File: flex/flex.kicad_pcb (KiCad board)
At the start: 2 copper layers, 126.3 x 91.6 mm, 91 parts, among them J1 Conn_01x04_Female, J2 Conn_01x05_Female, J3 Conn_01x03_Female, J4 Conn_01x06_Female, J5 Conn_01x03_Female, SW10 SW_Push, SW11 SW_Push, SW12 SW_Push, SW15 SW_Push, SW16 SW_Push, SW17 SW_Push, SW2 SW_Push, SW20 SW_Push, SW21 SW_Push, SW22 SW_Push, SW24 SW_Push, SW25 SW_Push, SW26 SW_Push, SW3 SW_Push, SW4 SW_Push, SW6 SW_Push, SW7 SW_Push, SW8 SW_Push

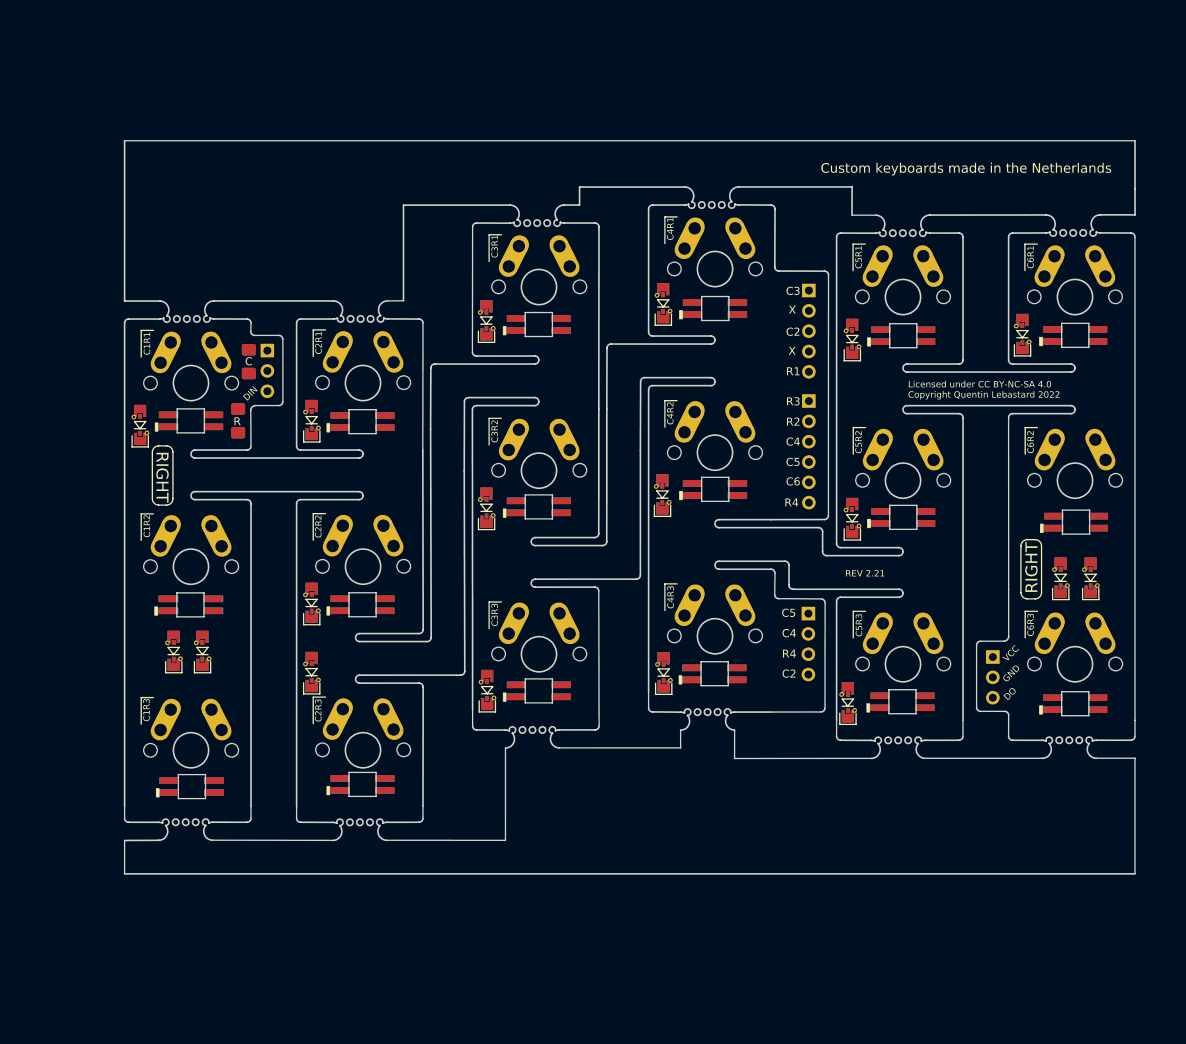
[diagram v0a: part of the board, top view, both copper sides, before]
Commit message: routing
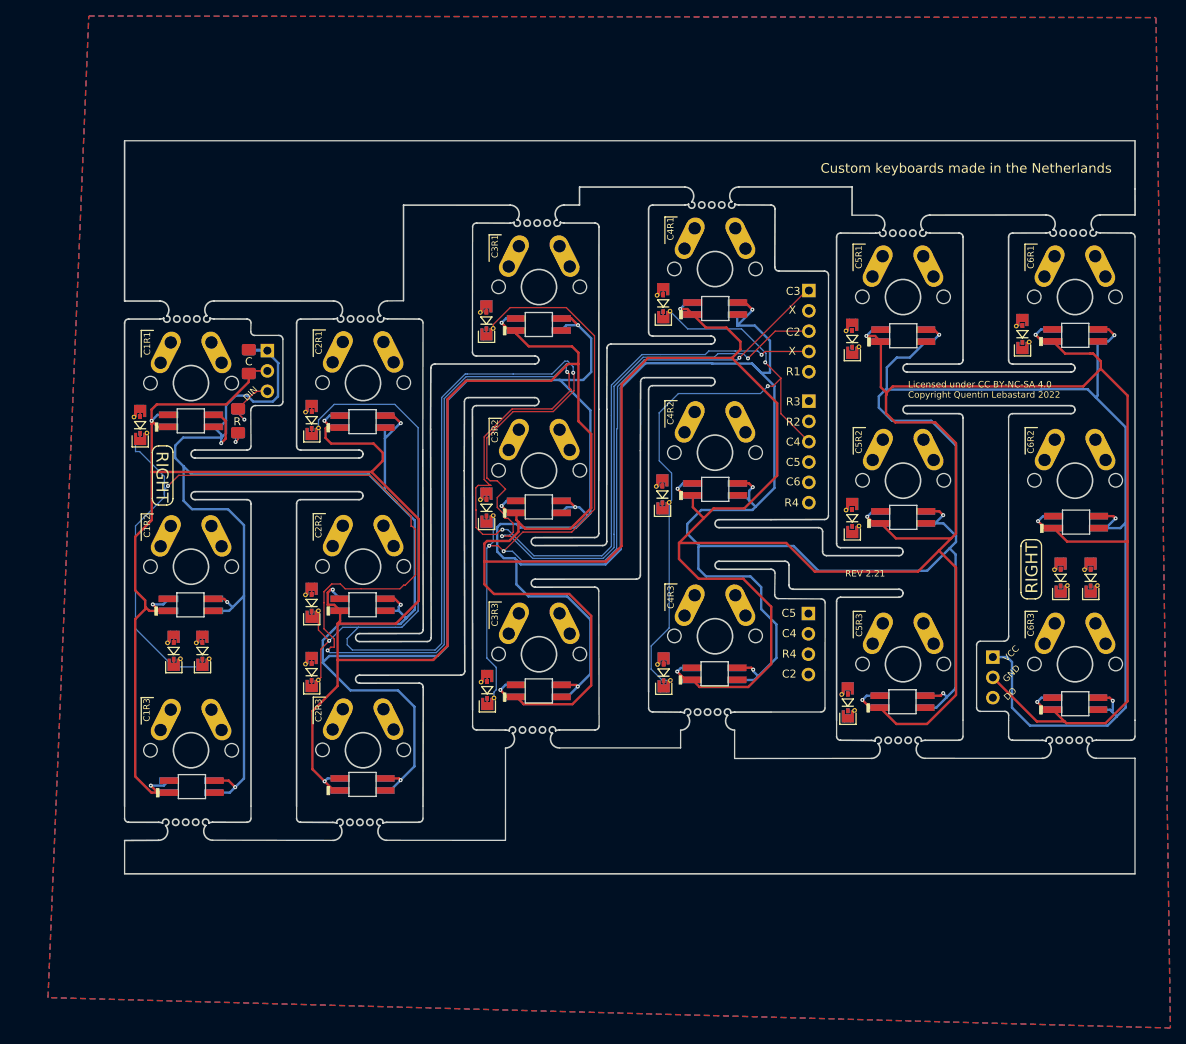
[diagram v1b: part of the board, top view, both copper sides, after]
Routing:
- net Gnd: track 0.00 -> 754.7 mm, vias 0 -> 18
- net Vcc: track 0.00 -> 725.8 mm, vias 0 -> 18
- net col1: track 0.00 -> 265.9 mm, vias 0 -> 5
- net col2: track 0.00 -> 227.6 mm, vias 0 -> 4
- net col3: track 0.00 -> 146.7 mm, vias 0 -> 3
- net col4: track 0.00 -> 87.0 mm, vias 0 -> 2
- net Din: track 0.00 -> 7.91 mm, vias 0 -> 1
- net Net-(D28-DIN): track 0.00 -> 2.57 mm, vias 0 -> 1
- net Net-(D9-A): track 0.00 -> 1.92 mm
- net Net-(D27-A): track 0.00 -> 1.92 mm
- net Net-(D20-A): track 0.00 -> 1.92 mm
- net Net-(D2-A): track 0.00 -> 1.92 mm
- net Net-(D19-A): track 0.00 -> 1.92 mm
- net Net-(D15-A): track 0.00 -> 1.92 mm
- net Net-(D13-A): track 0.00 -> 1.92 mm
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- added copper zone on B.Cu, net Gnd
- added copper zone on F.Cu, net Gnd

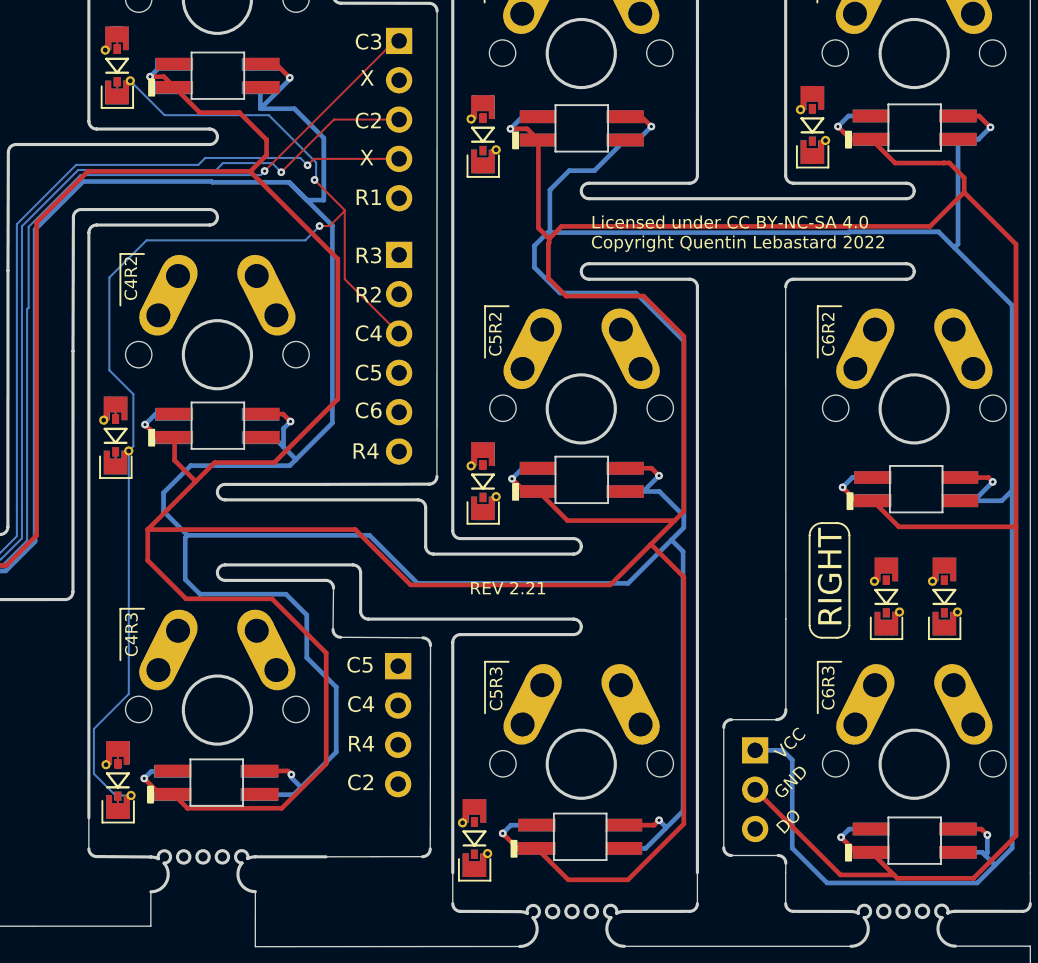
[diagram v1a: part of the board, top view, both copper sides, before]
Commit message: routing
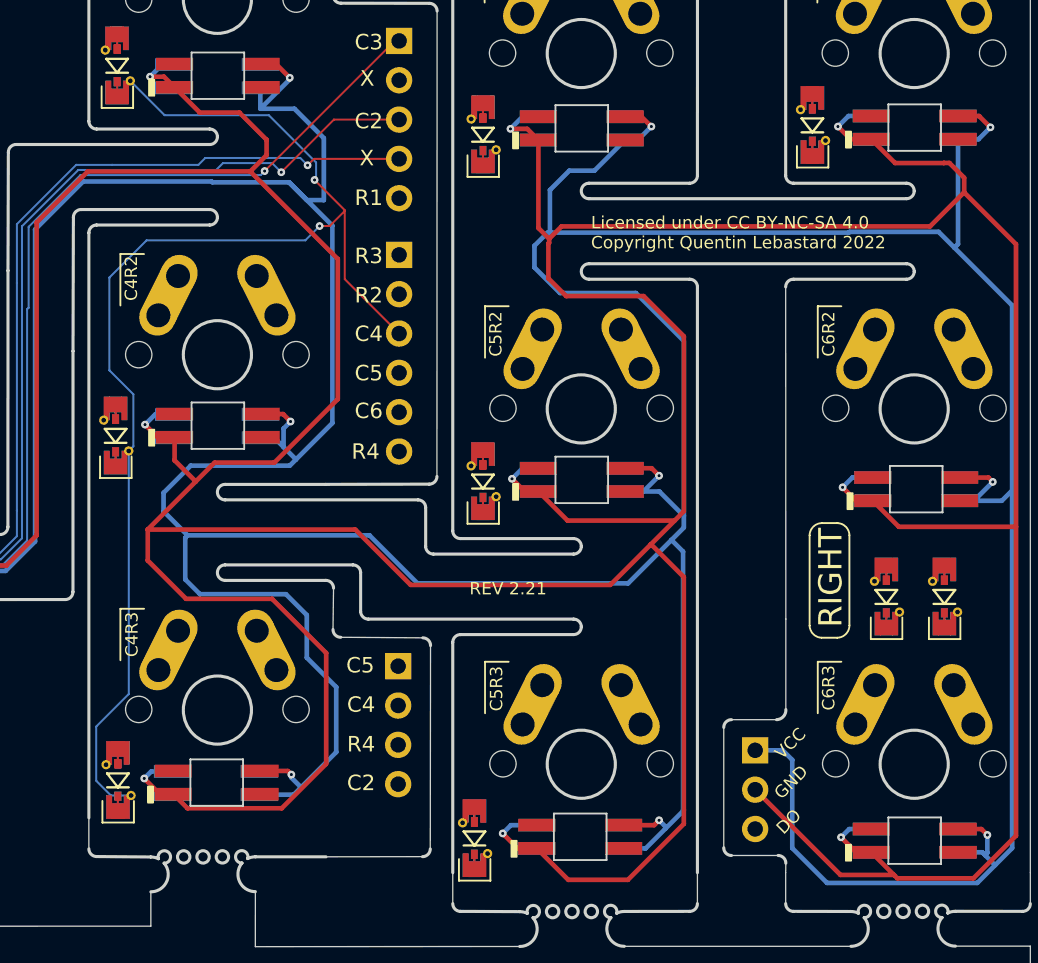
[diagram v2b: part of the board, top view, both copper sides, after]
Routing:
- net col6: track 0.00 -> 5.75 mm
- net col5: track 0.00 -> 5.75 mm
- net Net-(D36-A): track 0.00 -> 1.92 mm
- net Net-(D35-A): track 0.00 -> 1.92 mm
- net Net-(D32-A): track 0.00 -> 1.92 mm
- net Net-(D31-A): track 0.00 -> 1.92 mm
- net Net-(D16-A): track 0.00 -> 1.92 mm
- net Net-(D14-A): track 0.00 -> 1.92 mm
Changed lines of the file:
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@@
-	)
-	(segment
-		(start 101.25 114.05)
-		(end 102.65 115.45)
-		(width 0.13)
-		(layer "B.Cu")
-		(net 9)
 	)
 	(segment
@@
 	)
 	(segment
-		(start 103.5 108.9)
-		(end 101.25 111.15)
-		(width 0.13)
-		(layer "B.Cu")
-		(net 9)
-	)
-	(segment
 		(start 115.6 74.57168)
 		(end 115.6 75.6)
@@
 	)
 	(segment
+		(start 102.35 115.45)
+		(end 103.65 115.45)
+		(width 0.13)
+		(layer "B.Cu")
+		(net 9)
+	)
+	(segment
+		(start 103.5 108.9)
+		(end 101.4 111)
+		(width 0.13)
+		(layer "B.Cu")
+		(net 9)
+	)
+	(segment
+		(start 104.65 79.6)
+		(end 114.9 79.6)
+		(width 0.13)
+		(layer "B.Cu")
+		(net 9)
+	)
+	(segment
+		(start 101.4 111)
+		(end 101.4 114.5)
+		(width 0.13)
+		(layer "B.Cu")
+		(net 9)
+	)
+	(segment
 		(start 103.5 93.2)
 		(end 103.5 108.9)
@@
 	)
 	(segment
-		(start 104.65 79.6)
-		(end 114.9 79.6)
-		(width 0.13)
-		(layer "B.Cu")
-		(net 9)
-	)
-	(segment
-		(start 101.25 111.15)
-		(end 101.25 114.05)
-		(width 0.13)
-		(layer "B.Cu")
-		(net 9)
-	)
-	(segment
-		(start 102.65 115.45)
-		(end 103.65 115.45)
-		(width 0.13)
-		(layer "B.Cu")
-		(net 9)
-	)
-	(segment
 		(start 114.9 79.6)
 		(end 115.825735 78.674265)
@@
 		(layer "B.Cu")
 		(net 9)
+	)
+	(segment
+		(start 101.4 114.5)
+		(end 102.35 115.45)
+		(width 0.13)
+		(layer "B.Cu")
+		(net 9)
+	)
+	(segment
+		(start 125.8252 120.2105)
+		(end 125.8252 119.25275)
+		(width 0.13)
+		(layer "F.Cu")
+		(net 13)
+	)
+	(segment
+		(start 126.3752 73.80275)
+		(end 126.3752 74.7605)
+		(width 0.13)
+		(layer "F.Cu")
+		(net 13)
+	)
+	(segment
+		(start 126.3752 97.1605)
+		(end 126.3752 96.20275)
+		(width 0.13)
+		(layer "F.Cu")
+		(net 13)
+	)
+	(segment
+		(start 125.8252 120.2105)
+		(end 125.8252 119.25275)
+		(width 0.13)
+		(layer "B.Cu")
+		(net 13)
+	)
+	(segment
+		(start 126.3752 73.80275)
+		(end 126.3752 74.7605)
+		(width 0.13)
+		(layer "B.Cu")
+		(net 13)
+	)
+	(segment
+		(start 126.3752 96.20275)
+		(end 126.3752 97.1605)
+		(width 0.13)
+		(layer "B.Cu")
+		(net 13)
+	)
+	(segment
+		(start 147.65 74.15775)
+		(end 147.65 73.2)
+		(width 0.13)
+		(layer "F.Cu")
+		(net 14)
+	)
+	(segment
+		(start 152.4252 104.6105)
+		(end 152.4252 103.65275)
+		(width 0.13)
+		(layer "F.Cu")
+		(net 14)
+	)
+	(segment
+		(start 156.1752 104.6105)
+		(end 156.1752 103.65275)
+		(width 0.13)
+		(layer "F.Cu")
+		(net 14)
+	)
+	(segment
+		(start 156.1752 104.6105)
+		(end 156.1752 103.65275)
+		(width 0.13)
+		(layer "B.Cu")
+		(net 14)
+	)
+	(segment
+		(start 152.4252 103.65275)
+		(end 152.4252 104.6105)
+		(width 0.13)
+		(layer "B.Cu")
+		(net 14)
+	)
+	(segment
+		(start 147.65 73.2)
+		(end 147.65 74.15775)
+		(width 0.13)
+		(layer "B.Cu")
+		(net 14)
 	)
 	(segment
@@
 	)
 	(segment
+		(start 126.3752 71.70275)
+		(end 126.3752 70.745)
+		(width 0.13)
+		(layer "F.Cu")
+		(net 25)
+	)
+	(segment
+		(start 126.3752 70.745)
+		(end 126.3752 71.70275)
+		(width 0.13)
+		(layer "B.Cu")
+		(net 25)
+	)
+	(segment
 		(start 58.8 104.7)
 		(end 58.8 103.74225)
@@
 	)
 	(segment
+		(start 147.65 71.1)
+		(end 147.65 70.14225)
+		(width 0.13)
+		(layer "F.Cu")
+		(net 27)
+	)
+	(segment
+		(start 147.65 70.14225)
+		(end 147.65 71.1)
+		(width 0.13)
+		(layer "B.Cu")
+		(net 27)
+	)
+	(segment
 		(start 80.75 115.6)
 		(end 80.75 114.64225)
@@
 	)
 	(segment
+		(start 125.8252 117.15275)
+		(end 125.8252 116.195)
+		(width 0.13)
+		(layer "F.Cu")
+		(net 36)
+	)
+	(segment
+		(start 125.8252 117.15275)
+		(end 125.8252 116.195)
+		(width 0.13)
+		(layer "B.Cu")
+		(net 36)
+	)
+	(segment
+		(start 126.3752 94.10275)
+		(end 126.3752 93.145)
+		(width 0.13)
+		(layer "F.Cu")
+		(net 37)
+	)
+	(segment
+		(start 126.3752 93.145)
+		(end 126.3752 94.10275)
+		(width 0.13)
+		(layer "B.Cu")
+		(net 37)
+	)
+	(segment
+		(start 156.1752 101.55275)
+		(end 156.1752 100.595)
+		(width 0.13)
+		(layer "F.Cu")
+		(net 38)
+	)
+	(segment
+		(start 156.1752 101.55275)
+		(end 156.1752 100.595)
+		(width 0.13)
+		(layer "B.Cu")
+		(net 38)
+	)
+	(segment
+		(start 152.4252 101.55275)
+		(end 152.4252 100.595)
+		(width 0.13)
+		(layer "F.Cu")
+		(net 39)
+	)
+	(segment
+		(start 152.4252 100.595)
+		(end 152.4252 101.55275)
+		(width 0.13)
+		(layer "B.Cu")
+		(net 39)
+	)
+	(segment
